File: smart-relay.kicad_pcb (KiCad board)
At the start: 2 copper layers, 65.4 x 21.7 mm, 16 parts, among them IC1 TMCS1101A4BQDR, J1 Screw_Terminal_01x03, J2 Conn_01x04, K1 G5LE-1, Q1 BSS138K, U1 OPAMP, U2 ATtiny85-20PU

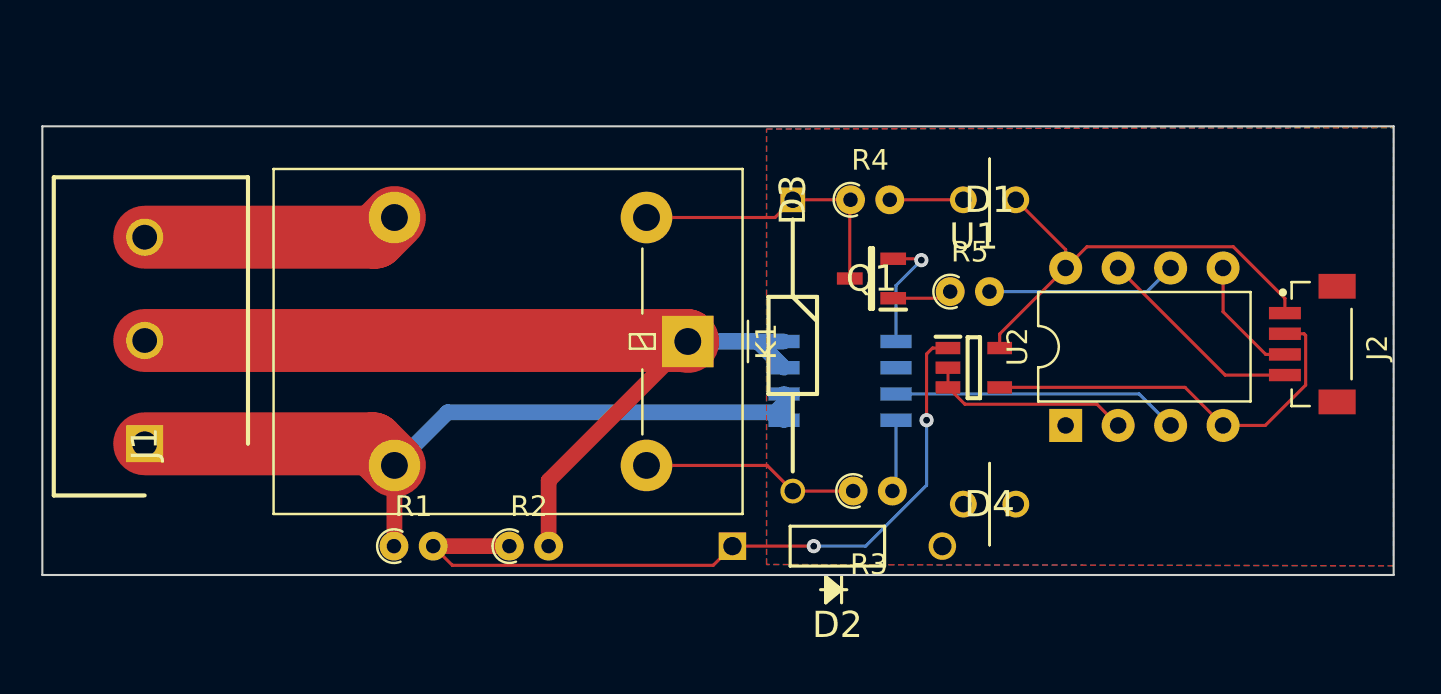
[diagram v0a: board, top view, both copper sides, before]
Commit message: don't remember
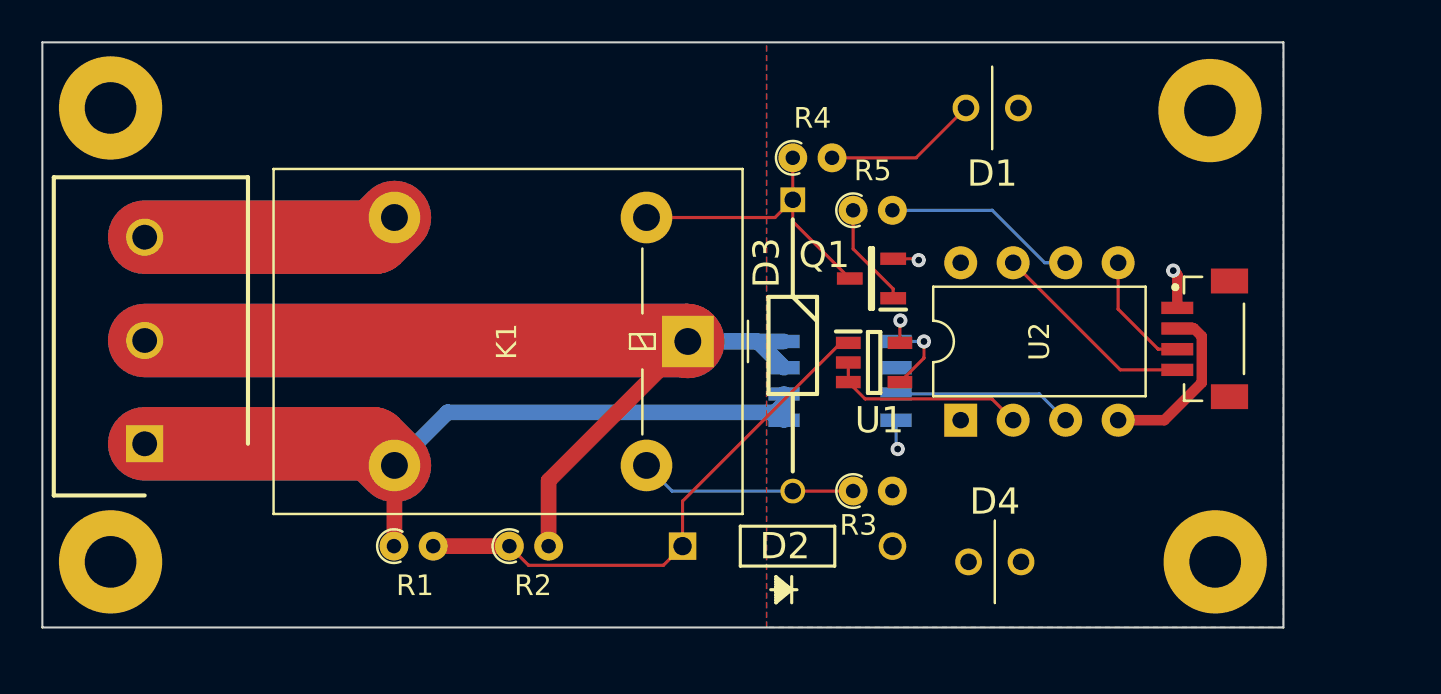
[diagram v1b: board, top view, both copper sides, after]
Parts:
- added REF**: MountingHole_2.5mm_Pad, MountingHole:MountingHole_2.5mm_Pad, F.Cu at (26.8, 47.2)
- added REF**: MountingHole_2.5mm_Pad, MountingHole:MountingHole_2.5mm_Pad, F.Cu at (26.8, 69.2)
- added REF**: MountingHole_2.5mm_Pad, MountingHole:MountingHole_2.5mm_Pad, F.Cu at (80.3, 69.2)
- added REF**: MountingHole_2.5mm_Pad, MountingHole:MountingHole_2.5mm_Pad, F.Cu at (80.0, 47.4)
- moved R5 6.13 mm to (62.7, 52.2)
- moved J2 5.21 mm to (79.8, 58.4)
- moved U2 5.09 mm to (67.9, 62.4)
- moved U1 4.83 mm to (63.8, 59.6)
- moved D1 4.45 mm to (68.2, 47.2)
- moved R4 3.45 mm to (59.8, 49.7)
- moved D4 2.81 mm to (68.3, 69.2)
- moved D2 2.41 mm to (54.5, 68.5)
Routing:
- net COM: track 48.8 -> 75.2 mm
- net +3V3: track 25.8 -> 4.43 mm, vias 0 -> 3
- net NC: track 37.8 -> 50.3 mm
- net NO: track 12.5 -> 25.0 mm
- net GND: track 25.7 -> 13.4 mm, vias 1 -> 2
- net Net-(D2-Pad2): track 37.1 -> 26.2 mm, vias 2 -> 0
- net ISENSE: track 13.9 -> 8.74 mm
- net Net-(D1-Pad1): track 3.56 -> 7.48 mm
- net Net-(Q1-Pad1): track 2.89 -> 5.06 mm
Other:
- board size 65.4 x 21.7 mm -> 60.1 x 28.3 mm
